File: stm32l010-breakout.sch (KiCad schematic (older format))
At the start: 29 parts, among them J1 SWD, J2 Left, J3 Right, Q1 BC847CDW1, SW1 Reset, U1 STM32L010K8Tx, Y1 32.768kHz

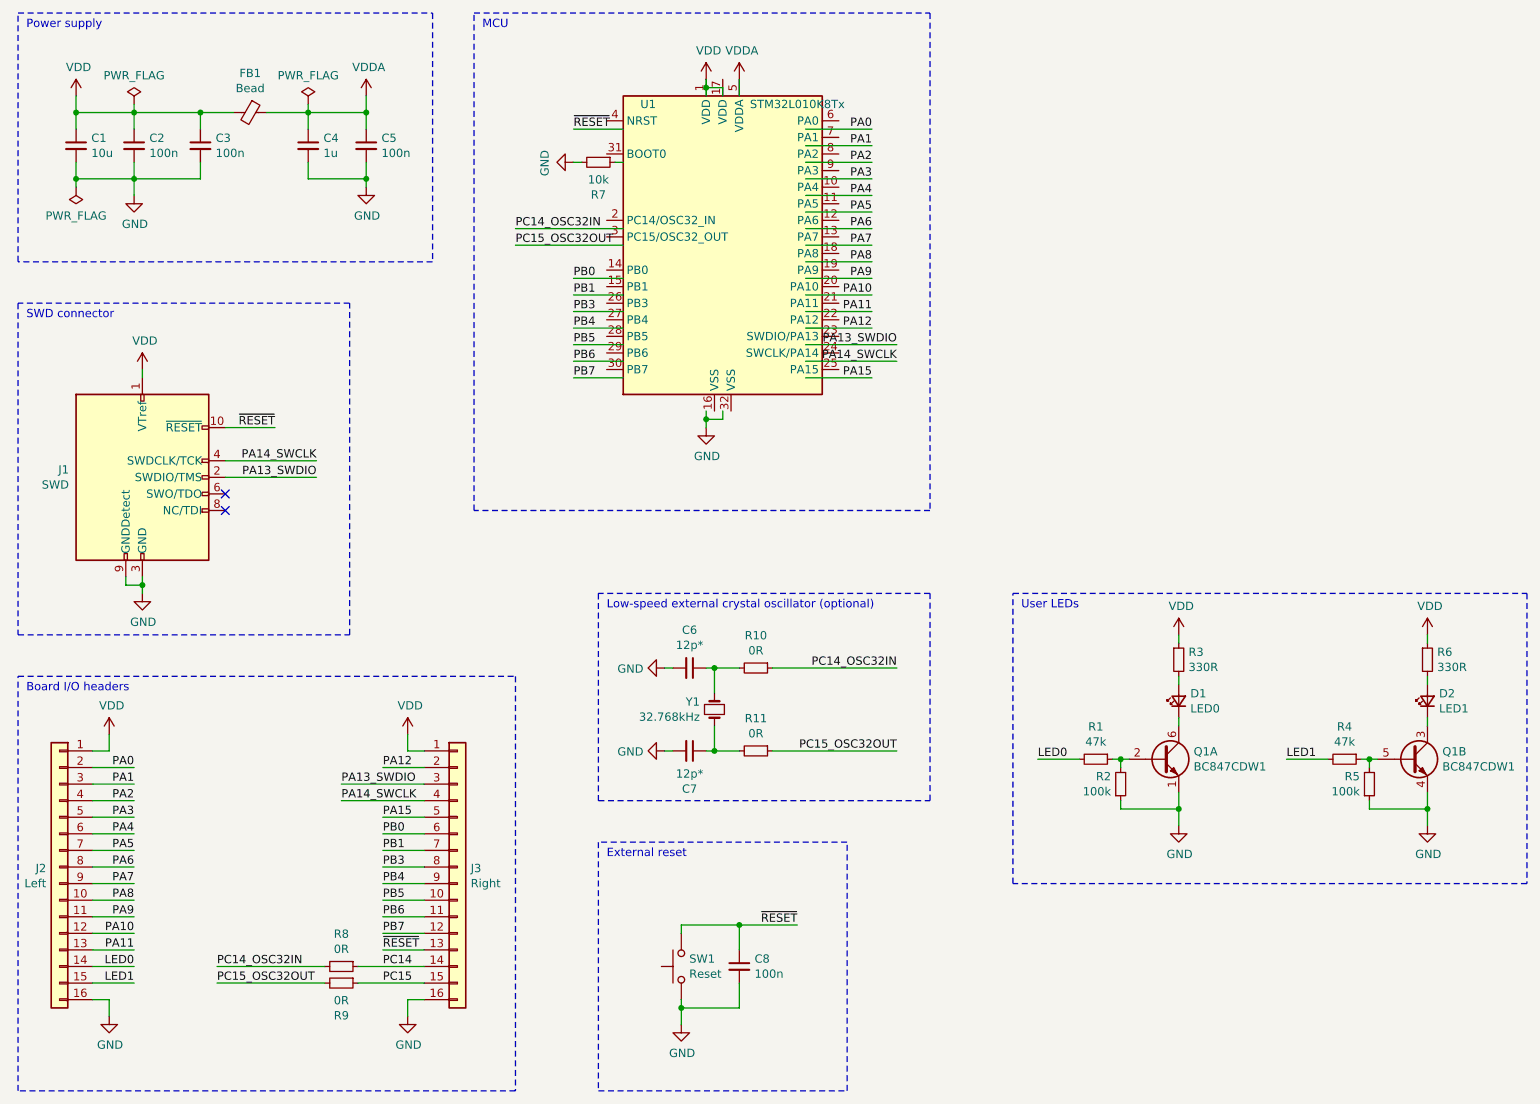
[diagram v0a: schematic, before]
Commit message: Schematic cleanup
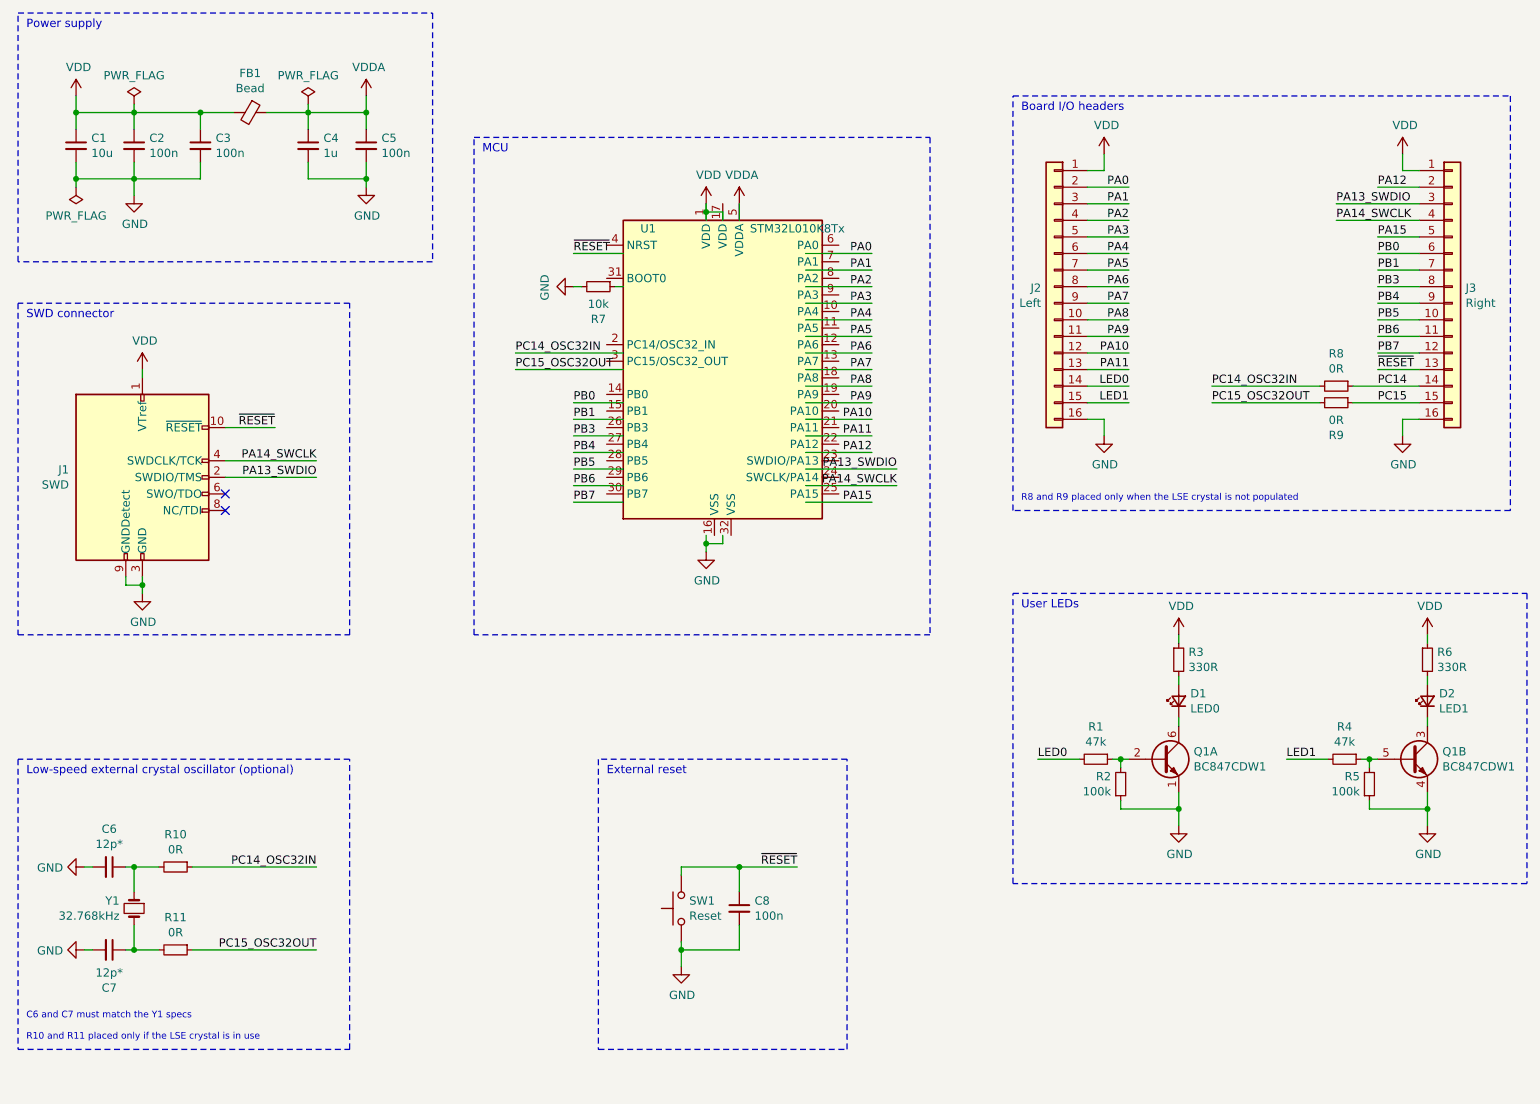
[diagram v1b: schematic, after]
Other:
- note added: "C6 and C7 must match the Y1 specs\n\nR10 and R11 placed only if the LSE crystal is in use"
- note added: "R8 and R9 placed only when the LSE crystal is not populated"
- moved on the sheet: C6, C7, C8, J2, J3, R10, R11, R7, R8, R9, SW1, U1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
